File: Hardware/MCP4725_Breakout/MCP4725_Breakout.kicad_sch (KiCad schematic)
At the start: 17 parts, among them J1 Conn_01x02, J2 I2C, U2 MCP4725

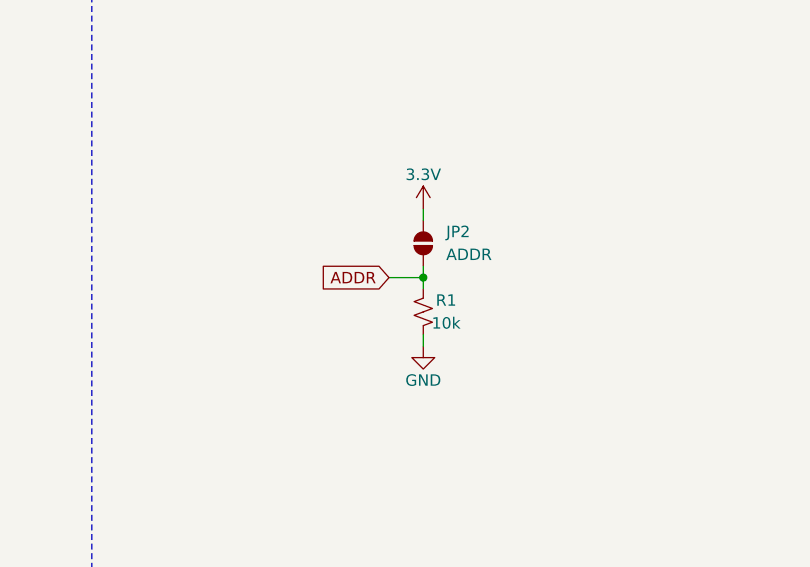
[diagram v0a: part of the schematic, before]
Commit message: Fixes jumpers on more time
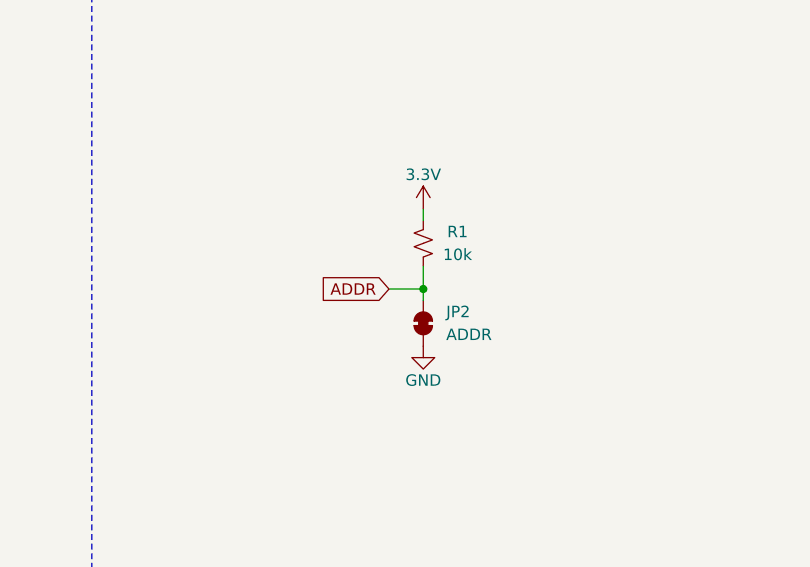
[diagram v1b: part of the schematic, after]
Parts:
- removed JP2: ADDR, SparkFun-Jumper:Jumper_2_NO, symbol SparkFun-Jumper:SolderJumper_2_Open
- added JP2: ADDR, SparkFun-Jumper:Jumper_2_NC_Trace, symbol SparkFun-Jumper:SolderJumper_2_Bridged
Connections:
- net 3.3V: now also R1.2
- net ADDR: now also R1.1, JP2.2 (B); no longer R1.2
- net GND: now also JP2.1 (A); no longer R1.1
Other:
- moved on the sheet: R1
